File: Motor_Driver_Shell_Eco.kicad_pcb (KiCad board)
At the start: 6 copper layers, 209 parts, among them J1 I2C EKRAN, J10 Conn_01x02, J11 USB_C_Receptacle, J12 Conn_01x02, J13 OUTSIDE LED, J2 HALL INPUT, J3 Conn_01x02, J4 Conn_01x02, J5 Conn_01x04, J6 Conn_01x06, J7 Conn_01x02, J8 Conn_01x03, J9 Conn_01x03, Q1 BC817, Q14 IAUS300N08S5N0, Q15 IAUS300N08S5N0, Q16 IAUS300N08S5N0, Q17 IAUS300N08S5N0, Q18 IAUS300N08S5N0, Q19 IAUS300N08S5N0, Q20 IAUS300N08S5N0, Q21 IAUS300N08S5N0, Q6 IAUS300N08S5N0, Q7 IAUS300N08S5N0, Q8 IAUS300N08S5N0, Q9 IAUS300N08S5N0, SW1 SW_Push, SW2 SW_Push, U1 STM32F205VGTx, U10 IRS21867S, U11 INA241A2, U12 TMP101, U13 INA241A2, U2 LM5017MR, U3 AP2204K-5.0, U4 XC6206 - 3V3, U5 INA241A2, U6 IRS21867S, U8 TJA1051T, U9 IRS21867S, Y1 8MHz

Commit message: changes to pcb and footprints
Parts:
- removed F1: Fuse, Fuse:Fuseholder_Littelfuse_445_030_series_5x30mm
- C1, C2, C3: footprint Capacitor_THT:CP_Radial_D18.0mm_P7.50mm -> Capacitor_THT:C_Radial_D16.0mm_H31.5mm_P7.50mm
- C10, C11, C12, C13, C14, C15, C16: footprint Capacitor_THT:C_Disc_D10.5mm_W5.0mm_P10.00mm -> Capacitor_SMD:C_0603_1608Metric_Pad1.08x0.95mm_HandSolder
- C17, C9: footprint Capacitor_THT:C_Disc_D10.5mm_W5.0mm_P10.00mm -> Capacitor_SMD:C_1210_3225Metric_Pad1.33x2.70mm_HandSolder
- C4, C5, C6: footprint Capacitor_SMD:C_1210_3225Metric_Pad1.33x2.70mm_HandSolder -> Capacitor_THT:C_Radial_D6.3mm_H11.0mm_P2.50mm
- L1: footprint Inductor_THT:L_Radial_D10.0mm_P5.00mm_Fastron_07P -> Inductor_SMD:L_1210_3225Metric_Pad1.42x2.65mm_HandSolder
- R3, R4, R5, R6: footprint Resistor_THT:R_Axial_DIN0207_L6.3mm_D2.5mm_P10.16mm_Horizontal -> Resistor_SMD:R_0603_1608Metric_Pad0.98x0.95mm_HandSolder
- moved H1 262.0 mm to (86.5, 57.2), turned to 0 degrees
- moved U3 261.8 mm to (99.8, 160.6), turned to 180 degrees
- moved R2 255.6 mm to (229.5, 175.9)
- moved C14 245.9 mm to (144.5, 206.9)
- moved D2 243.1 mm to (176.6, 162.9)
- moved C7 243.1 mm to (211.2, 161.6)
- moved C36 239.9 mm to (207.8, 209.4)
- moved C45 239.9 mm to (153.0, 165.6)
- moved D3 239.9 mm to (200.7, 203.4)
- moved J10 239.9 mm to (203.6, 185.2)
- moved J13 239.9 mm to (203.6, 197.3)
- moved J3 239.9 mm to (203.6, 173.1)
- moved J4 239.9 mm to (197.0, 203.4)
- moved NT1 239.9 mm to (179.0, 186.1)
- moved Q1 239.9 mm to (201.4, 207.6)
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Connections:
- C9 pad 2: GND -> -VDC
- H1 pad 1: Net-(F1-Pad1) -> Net-(H1-Pad1)
- S1 pad 1: Net-(F1-Pad2) -> Net-(H1-Pad1)
- S1 pad 2: Net-(F1-Pad2) -> Net-(H1-Pad1)
- S1 pad 3: Net-(F1-Pad2) -> Net-(H1-Pad1)
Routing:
- net -VDC: track 590.6 -> 945.7 mm, vias 555 -> 556
- net +VDC: track 408.5 -> 632.7 mm, vias 117 -> 167
- net +12V: track 9.03 -> 213.4 mm
- net Net-(F1-Pad2): track 40.3 -> 0.00 mm
- net ACCEL: track 0.00 -> 36.6 mm, vias 0 -> 1
- net Net-(H1-Pad1): track 0.00 -> 35.0 mm
- net REGEN: track 2.66 -> 31.8 mm
- net Net-(F1-Pad1): track 22.4 -> 0.00 mm
- net Net-(U2-SW): track 0.00 -> 11.6 mm
- net GND: track 63.7 -> 74.8 mm, vias 5 -> 11
- net Net-(U2-FB): track 0.00 -> 7.03 mm
- net Net-(U2-VCC): track 0.00 -> 6.97 mm, vias 0 -> 2
- net Net-(U2-BST): track 0.00 -> 6.46 mm, vias 0 -> 2
- net Net-(C15-Pad1): track 0.00 -> 5.79 mm
- net Net-(U2-RON): track 0.00 -> 1.98 mm
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- added copper zone on F.Cu, net +3V3
- added copper zone on In1.Cu, net GND
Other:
- board outline added: 207.2 x 164.4 mm

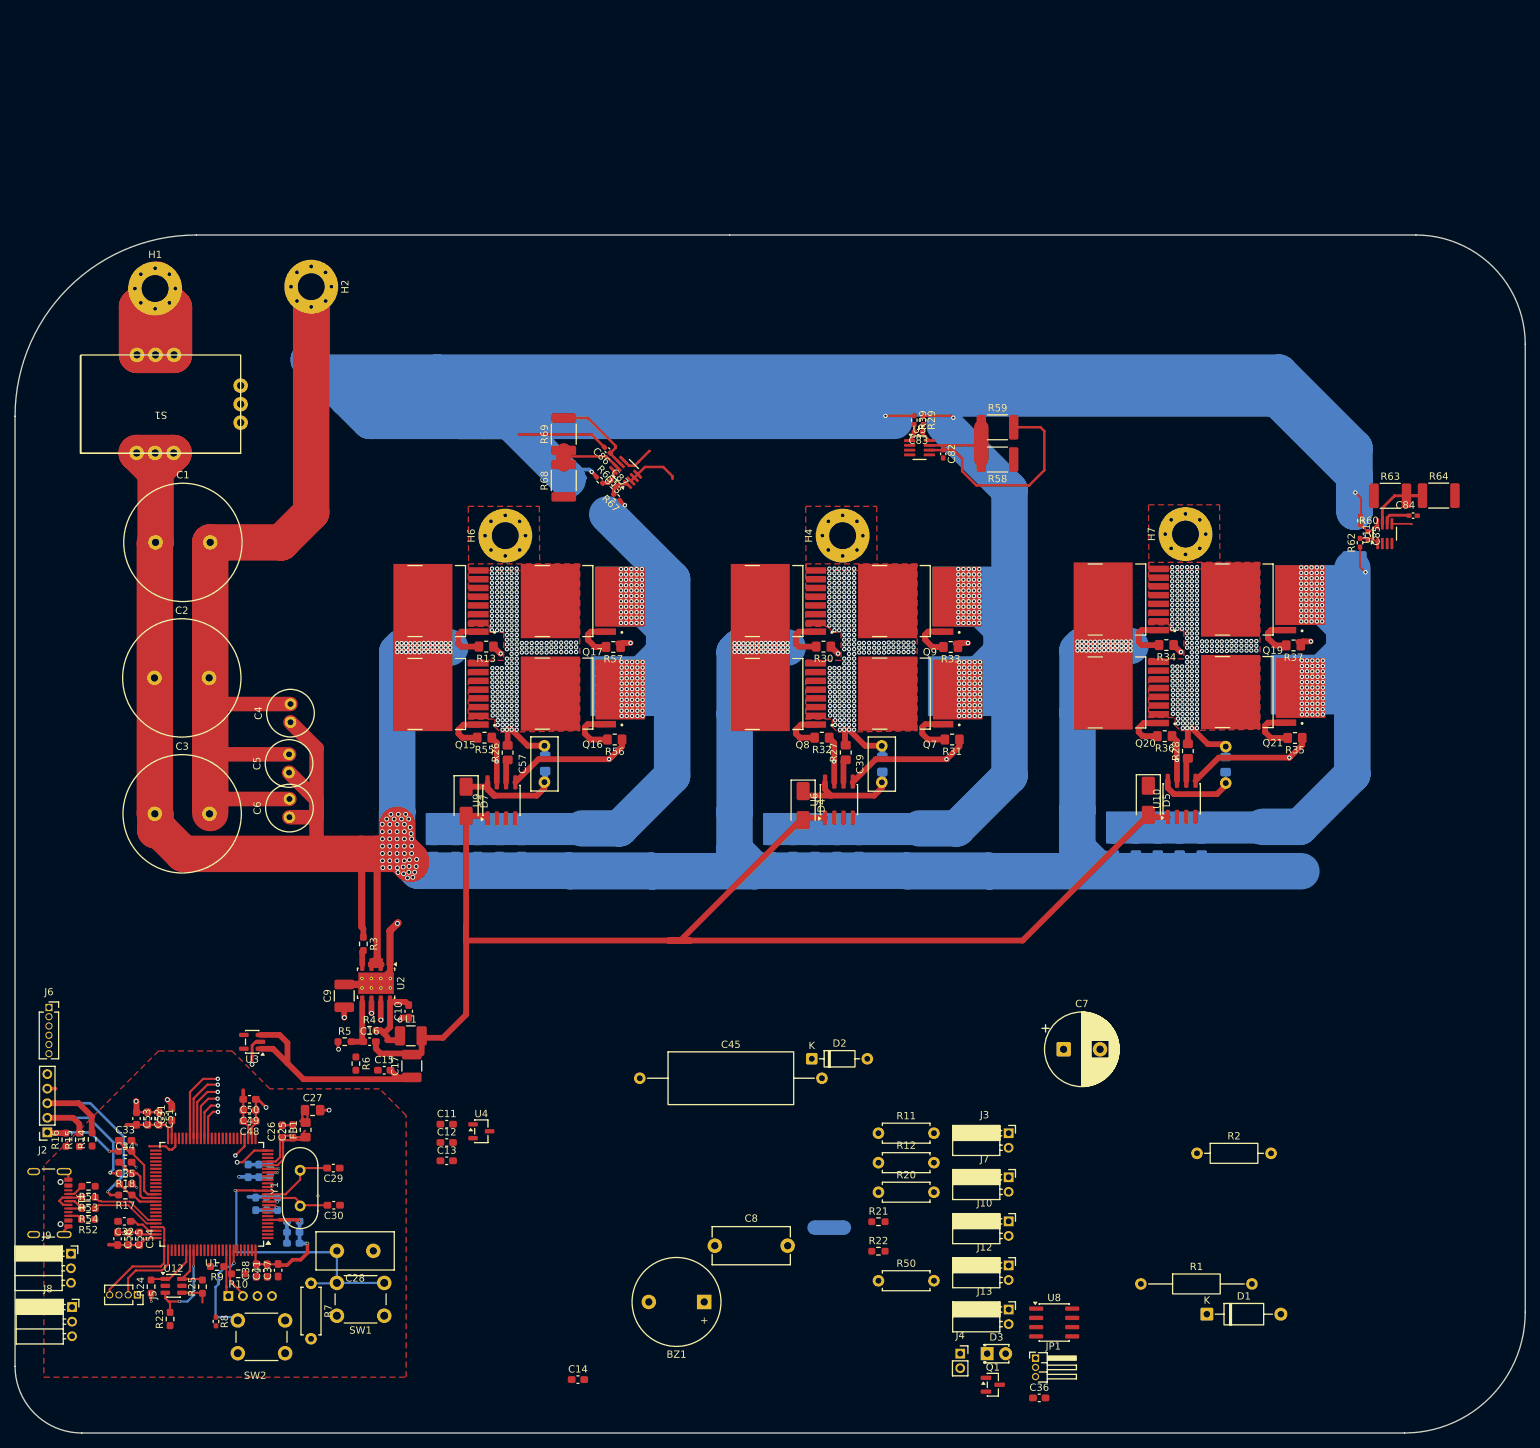
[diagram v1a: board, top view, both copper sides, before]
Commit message: LAST I HOPE
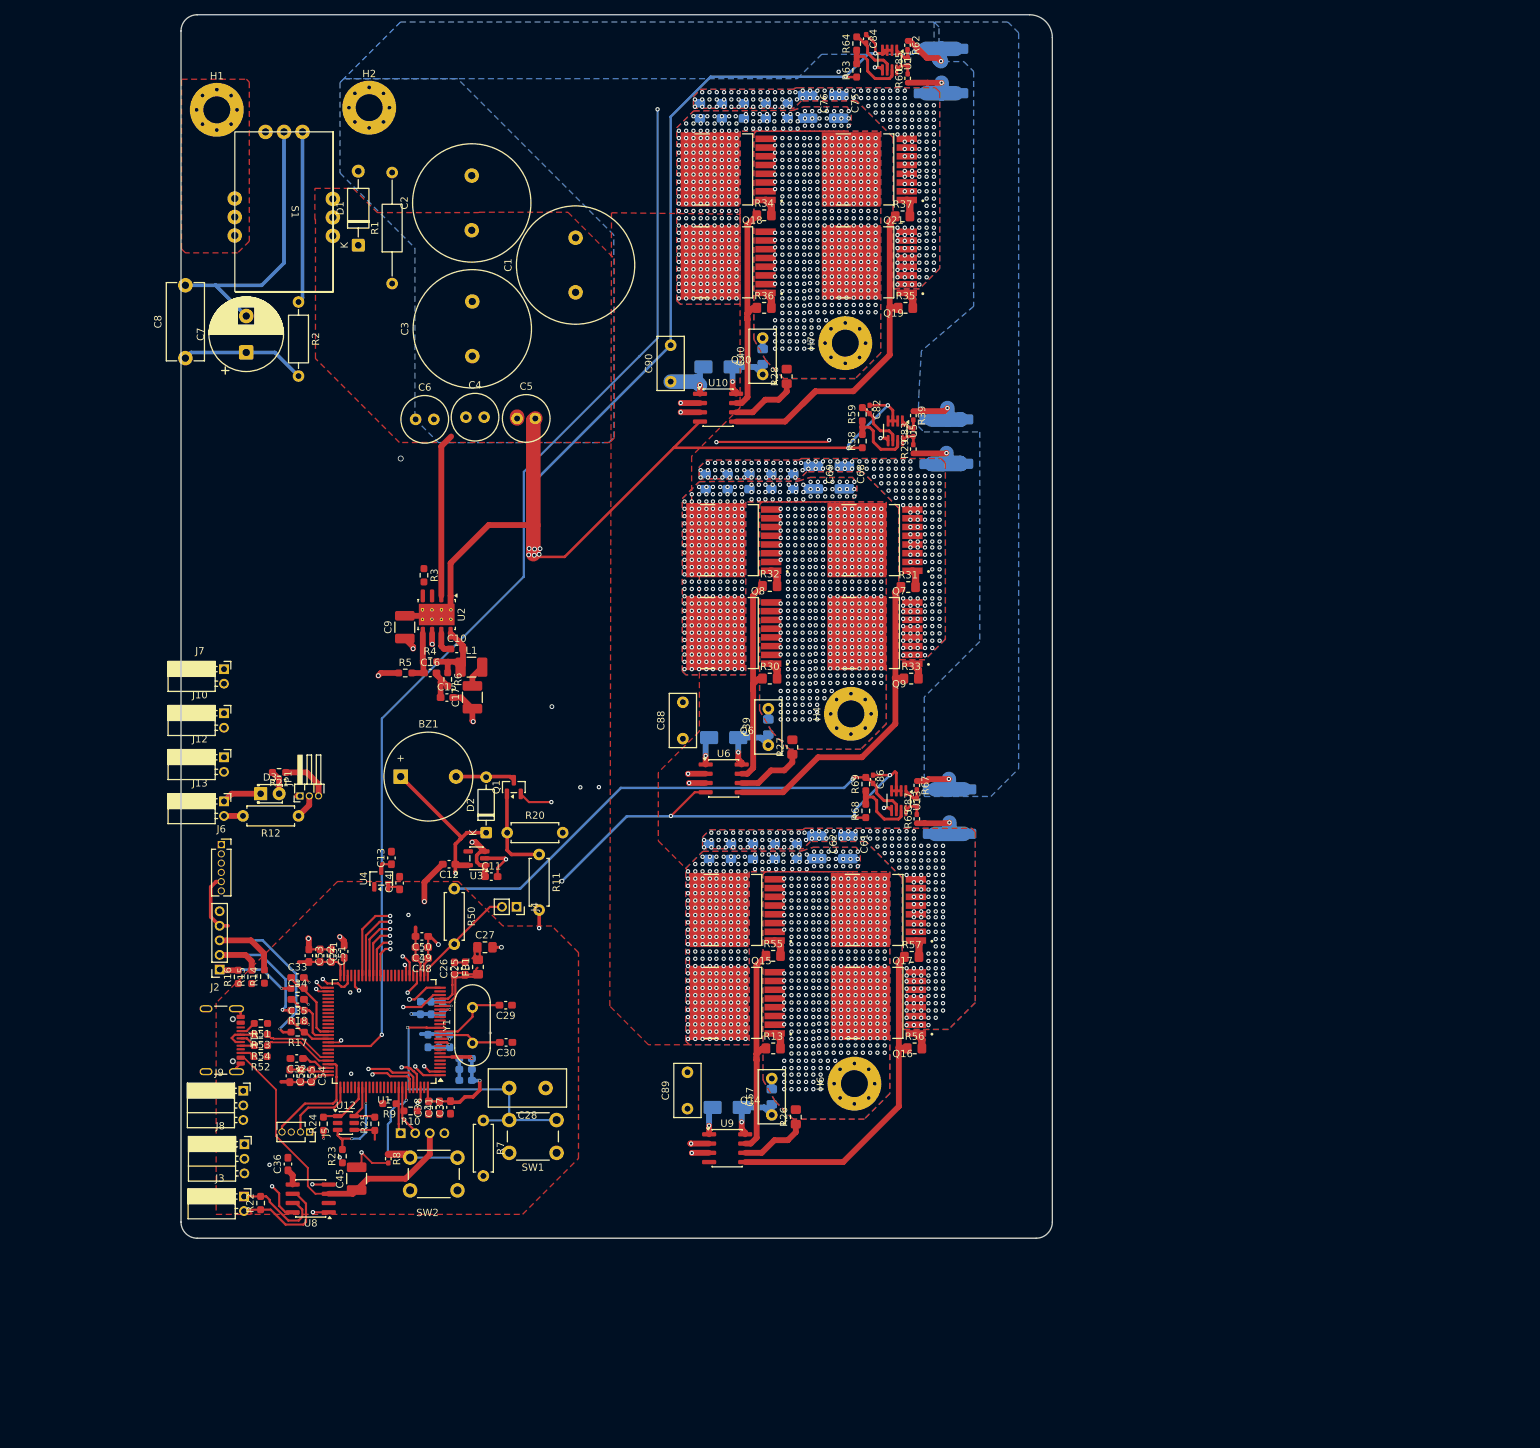
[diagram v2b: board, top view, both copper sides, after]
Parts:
- added C88: 4.7uF, Capacitor_THT:C_Rect_L7.2mm_W3.5mm_P5.00mm_FKS2_FKP2_MKS2_MKP2, F.Cu at (158.9, 119.0)
- added C89: 100nF, Capacitor_THT:C_Rect_L7.2mm_W3.5mm_P5.00mm_FKS2_FKP2_MKS2_MKP2, F.Cu at (159.5, 169.8)
- added C90: 4.7uF, Capacitor_THT:C_Rect_L7.2mm_W3.5mm_P5.00mm_FKS2_FKP2_MKS2_MKP2, F.Cu at (157.2, 70.0)
- added R70: 1mR, Resistor_SMD:R_2512_6332Metric_Pad1.40x3.35mm_HandSolder, B.Cu at (197.1, 78.2)
- added R71: 1mR, Resistor_SMD:R_2512_6332Metric_Pad1.40x3.35mm_HandSolder, B.Cu at (197.5, 129.0)
- added R72: 1mR, Resistor_SMD:R_2512_6332Metric_Pad1.40x3.35mm_HandSolder, B.Cu at (196.4, 27.4)
- C40, NT1: moved to F.Cu
- C45: footprint Capacitor_THT:C_Axial_L17.0mm_D7.0mm_P25.00mm_Horizontal -> Capacitor_SMD:C_1210_3225Metric_Pad1.33x2.70mm_HandSolder
- D4, D5, D7: moved to B.Cu
- R58, R59, R63, R64, R68, R69: footprint Resistor_SMD:R_1812_4532Metric_Pad1.30x3.40mm_HandSolder -> Resistor_SMD:R_0603_1608Metric_Pad0.98x0.95mm_HandSolder
- moved D1 187.3 mm to (114.3, 51.3), turned to 90 degrees
- moved R1 171.5 mm to (119.0, 56.5), turned to 90 degrees
- moved R2 169.9 mm to (106.2, 59.0), turned to -90 degrees
- moved C7 147.4 mm to (99.0, 66.0), turned to 90 degrees
- moved C8 141.8 mm to (90.6, 66.8), turned to 90 degrees
- moved J10 128.3 mm to (95.9, 115.5)
- moved J12 128.3 mm to (95.9, 121.5)
- moved J13 128.3 mm to (95.9, 127.6)
- moved J7 128.3 mm to (95.9, 109.4)
- moved JP1 127.0 mm to (106.4, 126.8), turned to 90 degrees
- moved D3 125.9 mm to (101.0, 126.5)
- moved C75 116.8 mm to (180.3, 32.2)
- moved C76 116.7 mm to (176.0, 32.2)
- moved C77 115.9 mm to (173.3, 32.8)
- moved C78 115.9 mm to (170.3, 32.8)
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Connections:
- U1 pad 31: Current_Sense_A -> Current Sense_A
- U1 pad 32: Current_Sense_B -> Current Sense_B
- U1 pad 46: unconnected-(U1-PE15-Pad46) -> PANIC STOP
- U1 pad 67: unconnected-(U1-PA8-Pad67) -> Current Sense_C
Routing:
- net -VDC: track 945.7 -> 115.5 mm, vias 556 -> 648
- net +VDC: track 632.7 -> 22.7 mm, vias 167 -> 828
- net GND: track 74.8 -> 465.3 mm, vias 11 -> 29
- net +5V: track 1.15 -> 211.2 mm, vias 0 -> 2
- net Current Sense_C: track 2.78 -> 184.2 mm, vias 0 -> 4
- net CSense_OUT_LES: track 0.00 -> 139.5 mm, vias 0 -> 1
- net Current Sense_B: track 0.00 -> 132.2 mm, vias 0 -> 4
- net HS_MOS_C: track 9.59 -> 101.7 mm, vias 1 -> 2
- net LS_MOS_C: track 10.9 -> 99.2 mm, vias 1 -> 2
- net Current Sense_A: track 4.68 -> 82.1 mm, vias 0 -> 3
- net BRAKE: track 0.00 -> 75.9 mm, vias 0 -> 1
- net CRUISE: track 0.00 -> 66.7 mm, vias 0 -> 1
- net STATUS_LED: track 0.00 -> 58.5 mm, vias 0 -> 1
- net /FET/LS_MOS_A: track 4.61 -> 60.0 mm, vias 1 -> 2
- net /FET/HS_MOS_A: track 5.82 -> 61.1 mm, vias 1 -> 2
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- added copper zone on B.Cu, net +VDC
- added copper zone on F.Cu, net +VDC
- added copper zone on In1.Cu, net +VDC
- added copper zone on In2.Cu, net +VDC
- added copper zone on In4.Cu, net +VDC
- added copper zone on B.Cu, net -VDC
- added copper zone on F.Cu, net -VDC
- added copper zone on In1.Cu, net -VDC
- added copper zone on In3.Cu, net -VDC
- added copper zone on In4.Cu, net -VDC
- added copper zone on B.Cu, net /FET/Phase_A_FET/PHASE_A
- added copper zone on In1.Cu, net /FET/Phase_A_FET/PHASE_A
- added copper zone on In2.Cu, net /FET/Phase_A_FET/PHASE_A
- added copper zone on In3.Cu, net /FET/Phase_A_FET/PHASE_A
- added copper zone on In4.Cu, net /FET/Phase_A_FET/PHASE_A
- added copper zone on B.Cu, net /FET/Phase_B_FET/PHASE_B
- added copper zone on In1.Cu, net /FET/Phase_B_FET/PHASE_B
- added copper zone on In2.Cu, net /FET/Phase_B_FET/PHASE_B
- added copper zone on In3.Cu, net /FET/Phase_B_FET/PHASE_B
- added copper zone on In4.Cu, net /FET/Phase_B_FET/PHASE_B
- added copper zone on B.Cu, net /FET/Phase_C_FET/PHASE_C
- added copper zone on F.Cu, net /FET/Phase_C_FET/PHASE_C
- added copper zone on In1.Cu, net /FET/Phase_C_FET/PHASE_C
- added copper zone on In2.Cu, net /FET/Phase_C_FET/PHASE_C
- added copper zone on In3.Cu, net /FET/Phase_C_FET/PHASE_C
- added copper zone on In4.Cu, net /FET/Phase_C_FET/PHASE_C
- added copper zone on F.Cu, net Net-(H1-Pad1)
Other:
- board size 207.2 x 164.4 mm -> 119.6 x 167.9 mm
- board text removed: "10R"
